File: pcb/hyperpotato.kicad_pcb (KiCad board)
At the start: 2 copper layers, 116.2 x 93.7 mm, 13 parts, among them SW1 SW_Push_45deg, SW10 SW_Push_45deg, SW11 SW_Push_45deg, SW12 SW_Push_45deg, SW13 SW_Push_45deg, SW2 SW_Push_45deg, SW3 SW_Push_45deg, SW4 SW_Push_45deg, SW5 SW_Push_45deg, SW6 SW_Push_45deg, SW7 SW_Push_45deg, SW8 SW_Push_45deg, SW9 SW_Push_45deg

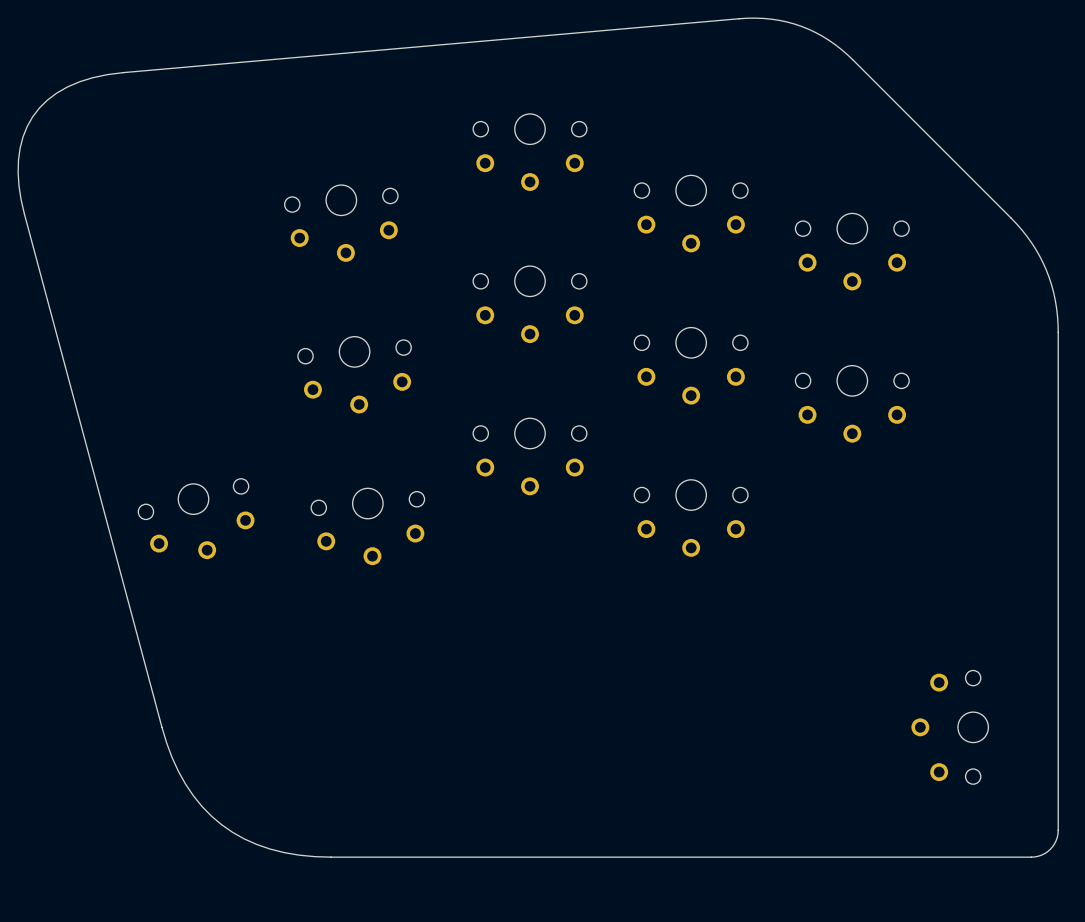
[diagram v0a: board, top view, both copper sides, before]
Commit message: Place test xiao footprint
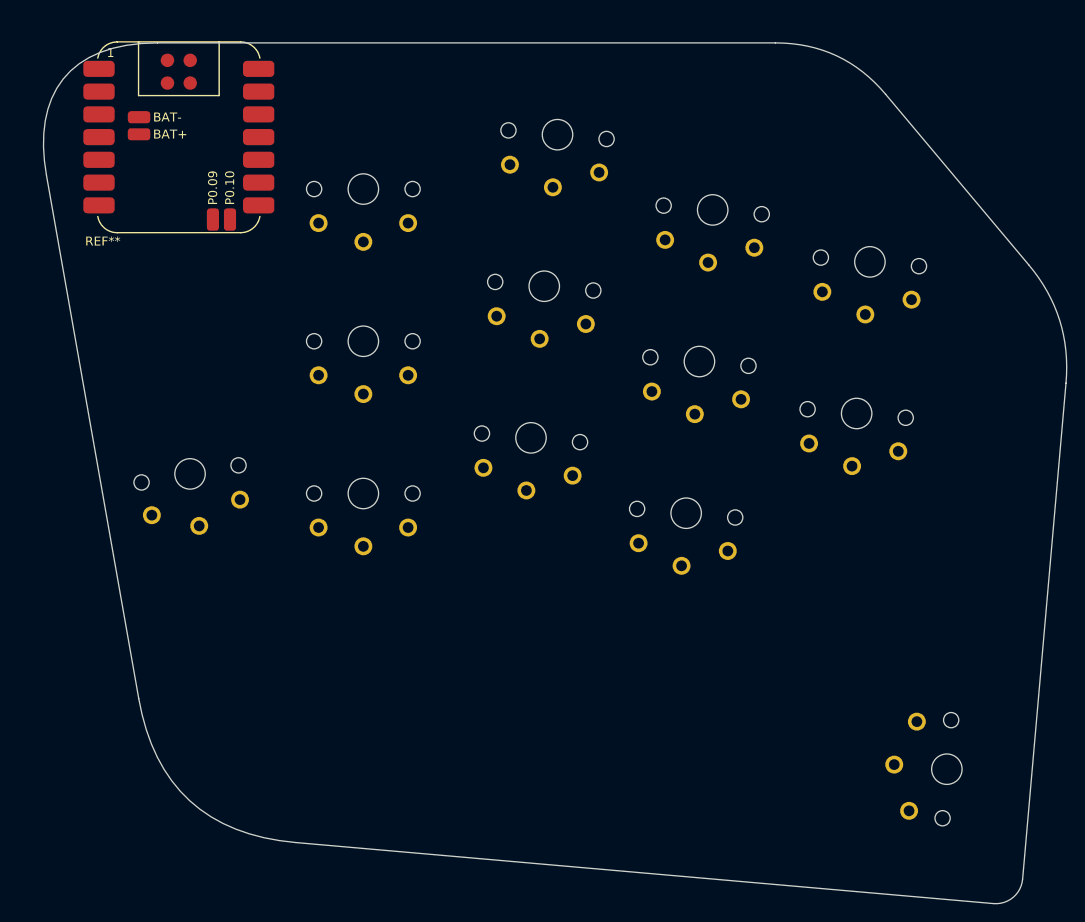
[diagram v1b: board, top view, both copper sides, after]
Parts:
- added REF**: Xiao_nRF52840_ACH_1, PCM_marbastlib-xp-promicroish:Xiao_nRF52840_AC_Reflow, F.Cu at (57.3, 64.5)
- moved SW13 5.52 mm to (143.1, 135.1), turned to -95 degrees
- moved SW4 4.20 mm to (134.5, 78.4), turned to -5 degrees
- moved SW9 3.68 mm to (133.0, 95.4), turned to -5 degrees
- moved SW3 3.23 mm to (117.0, 72.6), turned to -5 degrees
- moved SW2 3.13 mm to (99.6, 64.2), turned to -5 degrees
- moved SW5 2.84 mm to (58.6, 102.1), turned to 10 degrees
- moved SW1 2.76 mm to (77.9, 70.3), turned to 0 degrees
- moved SW8 2.29 mm to (115.5, 89.6), turned to -5 degrees
- moved SW12 2.10 mm to (114.0, 106.5), turned to -5 degrees
- moved SW7 1.68 mm to (98.2, 81.2), turned to -5 degrees
- moved SW6 1.54 mm to (77.9, 87.3), turned to 0 degrees
- moved SW10 1.23 mm to (77.9, 104.3), turned to 0 degrees
- moved SW11 0.50 mm to (96.7, 98.1), turned to -5 degrees
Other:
- board size 116.2 x 93.7 mm -> 114.3 x 96.1 mm
